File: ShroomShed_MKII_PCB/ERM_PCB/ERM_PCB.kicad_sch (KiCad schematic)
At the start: 18 parts, among them J1 Fan, J2 Humidifier, J3 Conn_01x04, Q1 BSS123, Q2 BSS123

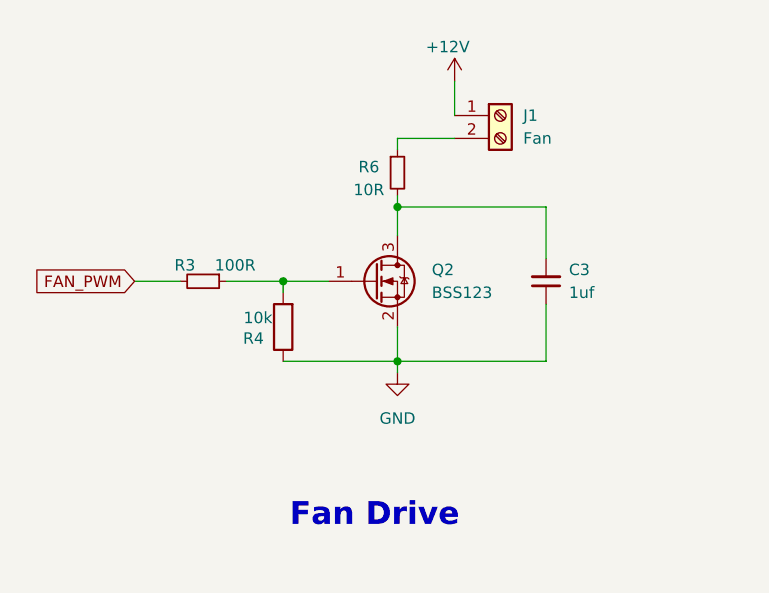
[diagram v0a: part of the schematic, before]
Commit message: Controller V2.2 ordered
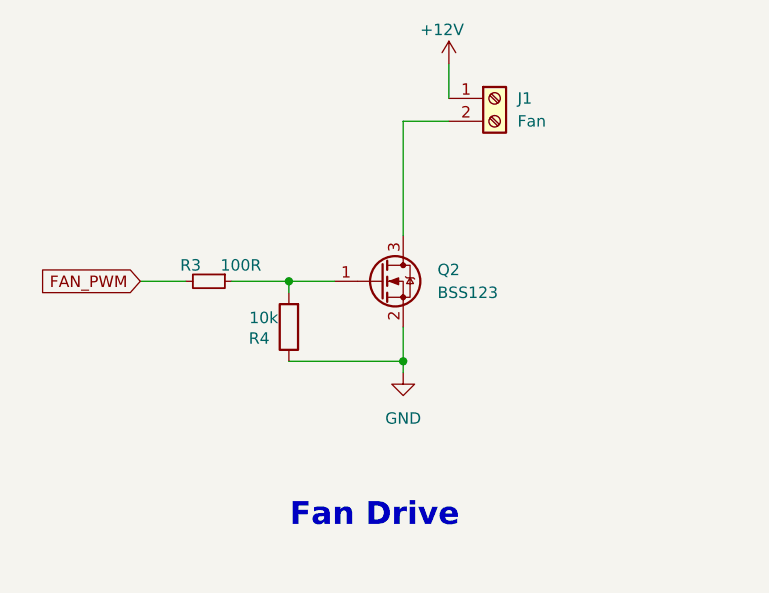
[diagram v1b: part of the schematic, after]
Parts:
- removed C3: 1uf, Capacitor_SMD:C_0603_1608Metric, symbol Device:C_Small
- removed R6: 10R, Resistor_SMD:R_0805_2012Metric, symbol Device:R_Small
- R1, R3: DESCRIPTION C22775 -> (none)
- R2, R4, R5: DESCRIPTION C25804 -> (none)
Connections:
- net at J1.2 (Pin_2): now also Q2.3 (D)
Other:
- moved on the sheet: J1, Q2, R3, R4
